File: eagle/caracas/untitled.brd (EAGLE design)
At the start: 100 x 49.5 mm, 26 parts, among them IC1 4027N, Q1 IRFP250, X1 22-23-2021, X2 22-23-2021, X3 22-23-2041, X4 22-23-2041, X5 22-23-2021, X6 22-23-2021

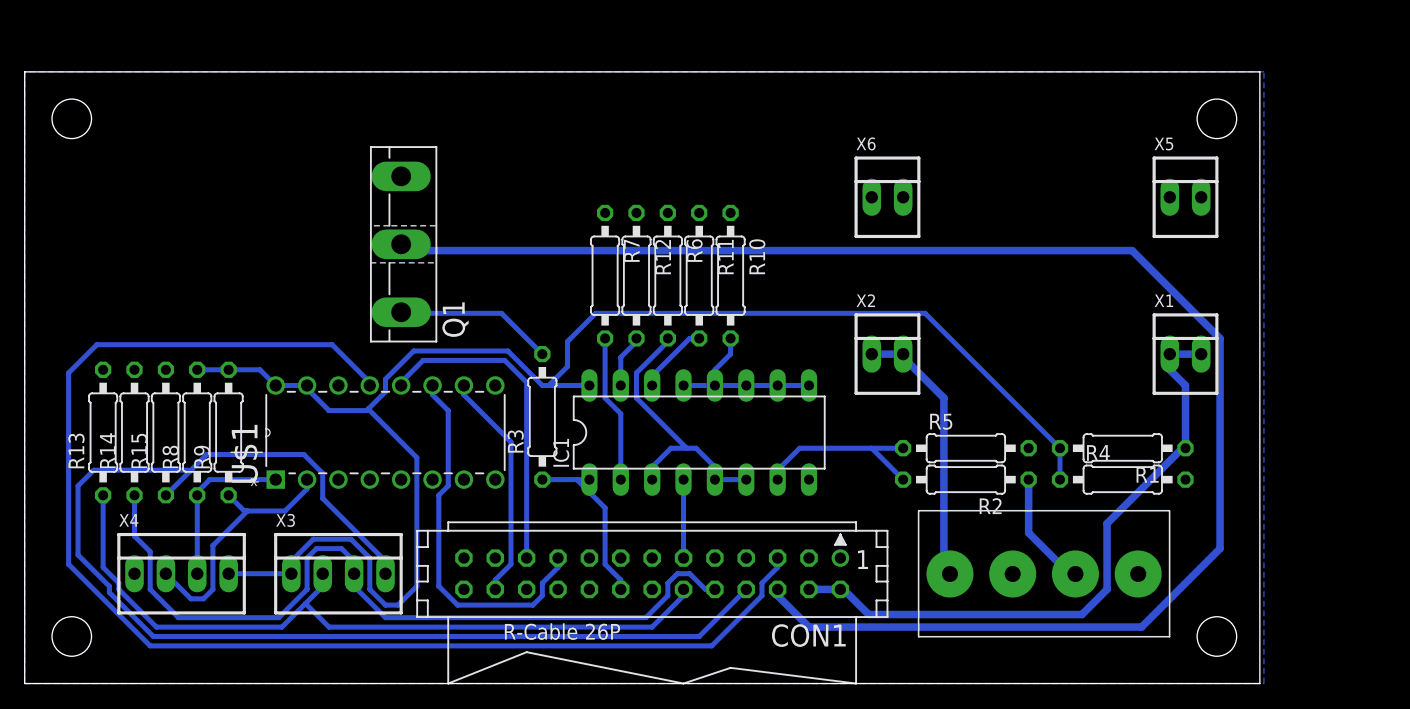
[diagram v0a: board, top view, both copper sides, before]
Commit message: Schematic and board finished (at least R1)
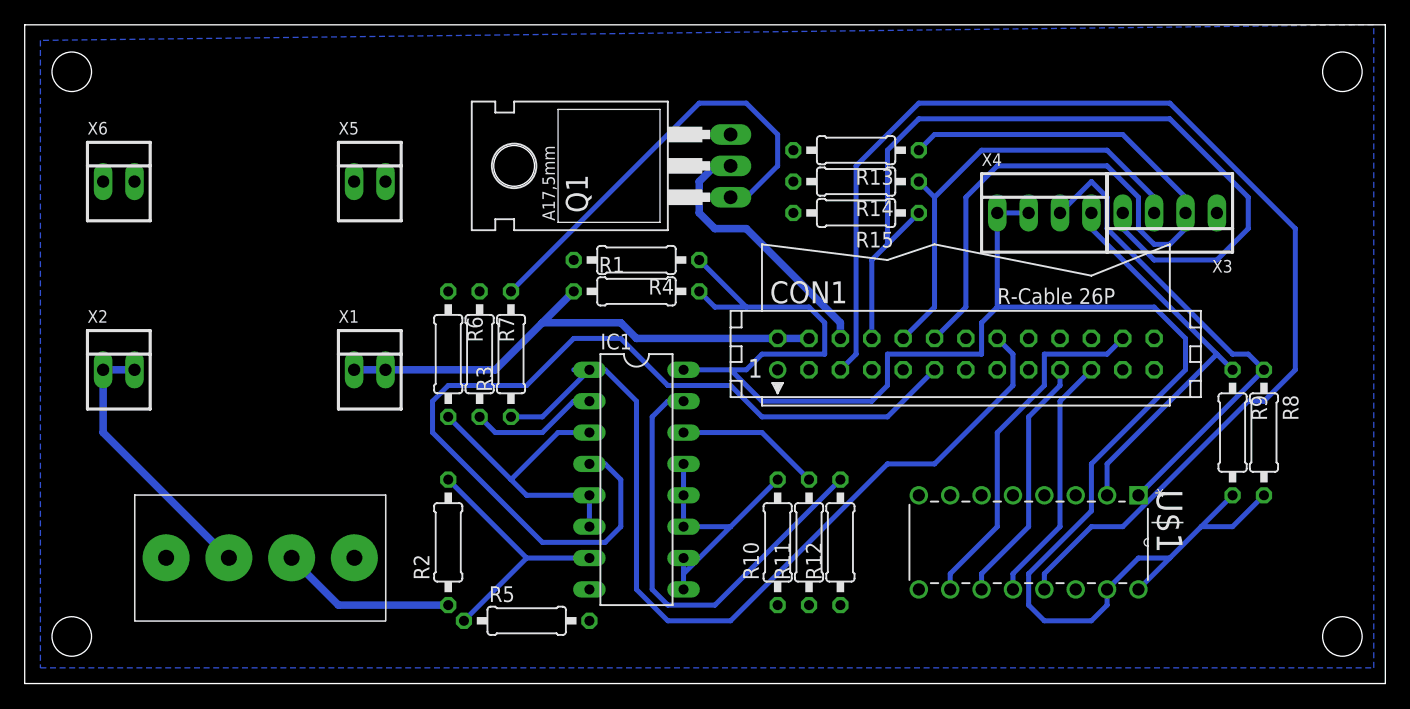
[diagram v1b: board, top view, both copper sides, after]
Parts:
- Q1: value IRFP250 -> IRLZ44Z; device transistor-power:TO-247AD-V -> transistor-power:TO220BH
- moved R8 86.4 mm to (100.3, 20.3), turned to 270 degrees
- moved R9 81.3 mm to (97.8, 20.3), turned to 270 degrees
- moved X4 75.7 mm to (82.5, 38.1)
- moved X3 73.4 mm to (92.7, 38.1), turned to 180 degrees
- moved X1 66.1 mm to (27.9, 25.4)
- moved X5 66.1 mm to (27.9, 40.6)
- moved R13 65.1 mm to (67.3, 43.2), turned to 180 degrees
- moved U$2 63.5 mm to (19.1, 10.2), turned to 0 degrees
- moved X2 62.2 mm to (7.62, 25.4)
- moved X6 62.2 mm to (7.62, 40.6)
- moved R14 61.9 mm to (67.3, 40.6), turned to 180 degrees
- moved R15 58.6 mm to (67.3, 38.1), turned to 180 degrees
- moved R4 43.2 mm to (49.5, 34.3), turned to 180 degrees
- moved R2 42.2 mm to (34.3, 11.4), turned to 90 degrees
- moved R1 41.4 mm to (49.5, 31.8), turned to 0 degrees
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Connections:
- net +12V_IGN: now also U$2.P$4; no longer U$2.P$3
- net +3.3V: now also X4.1, X4.2; no longer X3.1, X4.4
- net ANA_1: now also X4.4; no longer X4.2
- net GND: no longer X4.1
- net VCC: now also U$2.P$3; no longer U$2.P$2
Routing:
- net +5V_SW_GND: track 126.5 -> 22.0 mm
- net SUICIDE: track 6.35 -> 75.8 mm
- net POWER_STATE: track 14.2 -> 73.1 mm
- net N$13: track 4.34 -> 37.0 mm
- net N$7: track 98.8 -> 68.3 mm
- net N$8: track 64.7 -> 36.5 mm
- net ANA_0: track 13.4 -> 39.7 mm
- net N$1: track 12.9 -> 36.4 mm
- net +3.3V: track 126.4 -> 144.9 mm
- net ANA_1: track 20.8 -> 32.5 mm
- net N$6: track 18.6 -> 29.1 mm
- net N$5: track 30.0 -> 20.4 mm
- net +5V: track 50.7 -> 42.5 mm
- net N$12: track 14.5 -> 22.2 mm
- net N$3: track 106.5 -> 98.8 mm
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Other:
- board size 100 x 49.5 mm -> 110.2 x 53.3 mm
